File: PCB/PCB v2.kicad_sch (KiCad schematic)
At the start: 0 parts

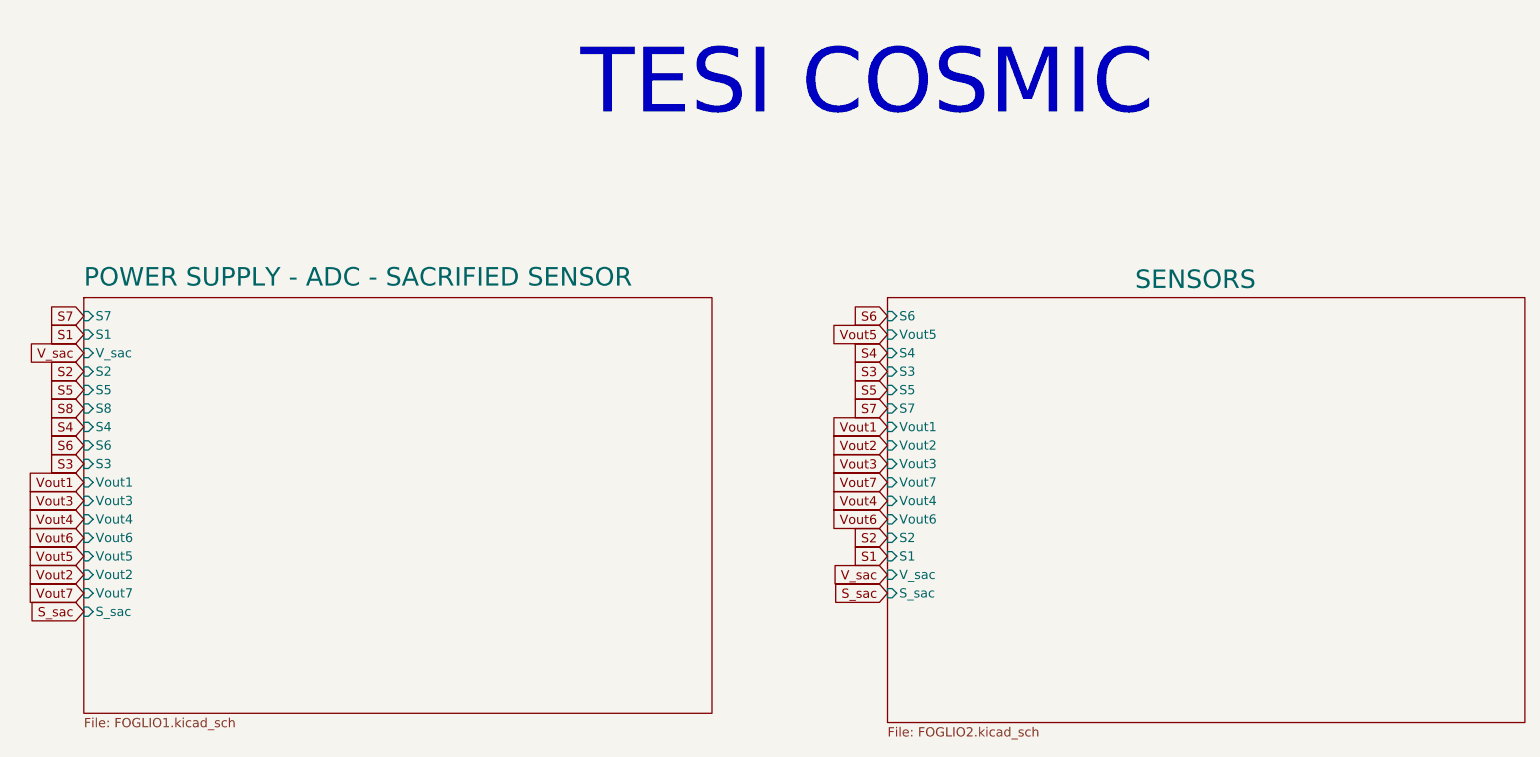
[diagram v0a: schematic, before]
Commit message: Modifiche accordate fatte
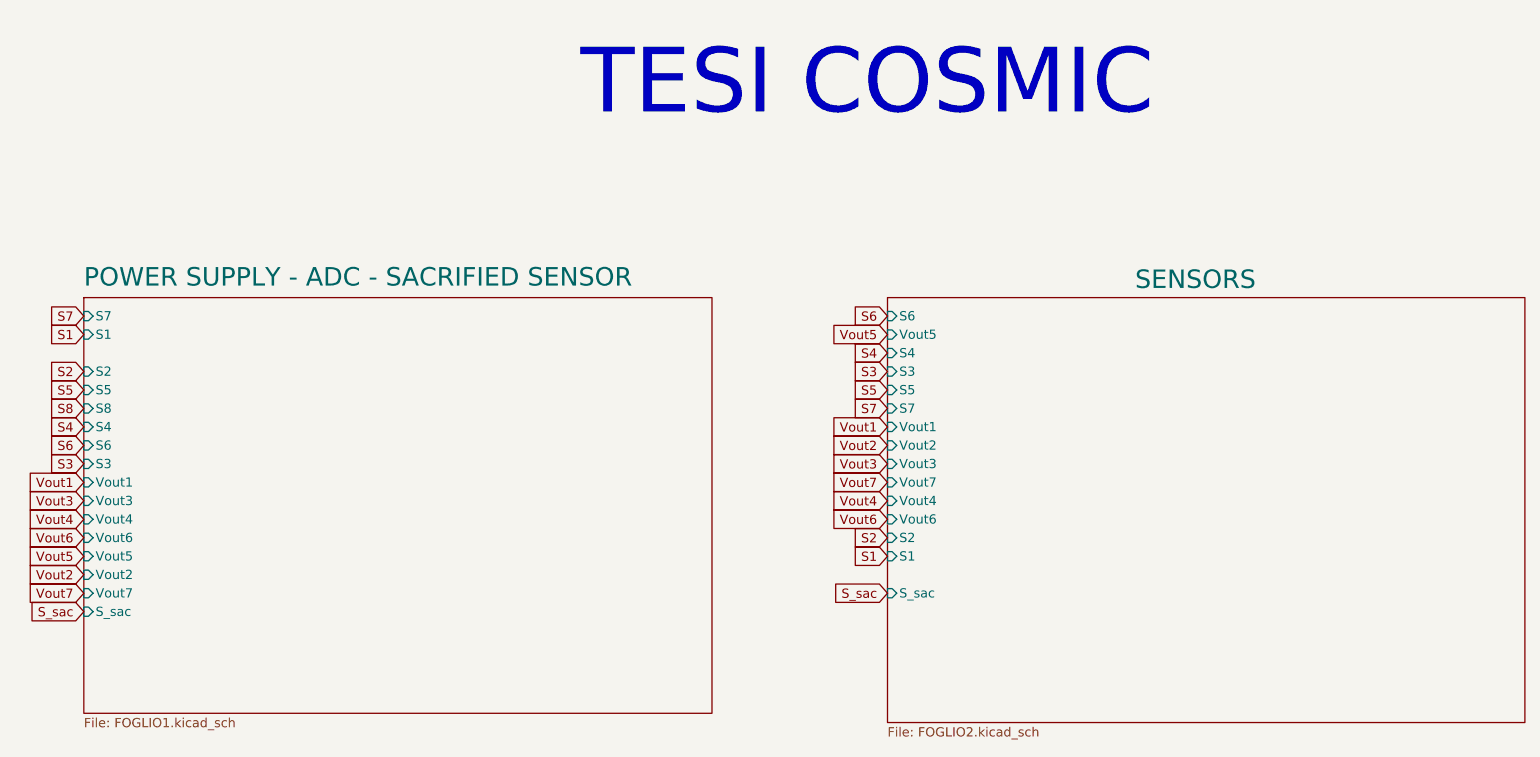
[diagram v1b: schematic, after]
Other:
- sheet POWER SUPPLY - ADC - SACRIFIED SENSOR ports: added none; removed V_sac
- sheet SENSORS ports: added none; removed V_sac
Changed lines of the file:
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@@
-		)
-	)
-	(global_label "V_sac"
-		(shape input)
-		(at 151.13 90.17 180)
-		(fields_autoplaced yes)
-		(effects
-			(font
-				(size 1.27 1.27)
-			)
-			(justify right)
-		)
-		(property "Intersheetrefs" "${INTERSHEET_REFS}"
-			(at 142.8229 90.17 0)
-			(hide yes)
-			(show_name no)
-			(do_not_autoplace no)
-			(effects
-				(font
-					(size 1.27 1.27)
-				)
-				(justify right)
-			)
 		)
 	)
@@
 		(property "Intersheetrefs" "${INTERSHEET_REFS}"
 			(at 145.7258 85.09 0)
-			(hide yes)
-			(show_name no)
-			(do_not_autoplace no)
-			(effects
-				(font
-					(size 1.27 1.27)
-				)
-				(justify right)
-			)
-		)
-	)
-	(global_label "V_sac"
-		(shape input)
-		(at 40.64 59.69 180)
-		(fields_autoplaced yes)
-		(effects
-			(font
-				(size 1.27 1.27)
-			)
-			(justify right)
-		)
-		(property "Intersheetrefs" "${INTERSHEET_REFS}"
-			(at 32.3329 59.69 0)
 			(hide yes)
 			(show_name no)
@@
 			)
 		)
-		(pin "V_sac" input
-			(at 151.13 90.17 180)
-			(effects
-				(font
-					(size 1.27 1.27)
-				)
-				(justify left)
-			)
-		)
 		(pin "S_sac" input
 			(at 151.13 92.71 180)
@@
 			(effects
 				(font
-					(size 1.27 1.27)
-				)
-				(justify left)
-			)
-		)
-		(pin "V_sac" input
-			(at 40.64 59.69 180)
-			(effects
-				(font
